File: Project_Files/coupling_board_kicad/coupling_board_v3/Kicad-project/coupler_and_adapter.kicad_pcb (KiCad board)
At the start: 2 copper layers, 98.8 x 70 mm, 95 parts, among them IC1 ISO6741DWR, IC2 ISO6740FDWR, IC3 ISO6740FDWR, J1 Conn_02x04_Odd_Even, J1 Molex Microfit, J10 Conn_02x12_Odd_Even, J2 Conn_02x04_Odd_Even, J2 Conn_02x12_Odd_Even, J3 Conn_02x04_Odd_Even, J3 Molex6, J4 Conn_02x12_Odd_Even, J5 DB25_Socket, J6 DB25_Socket, J7 Molex Microfit, J8 Molex Microfit, J9 Molex Microfit

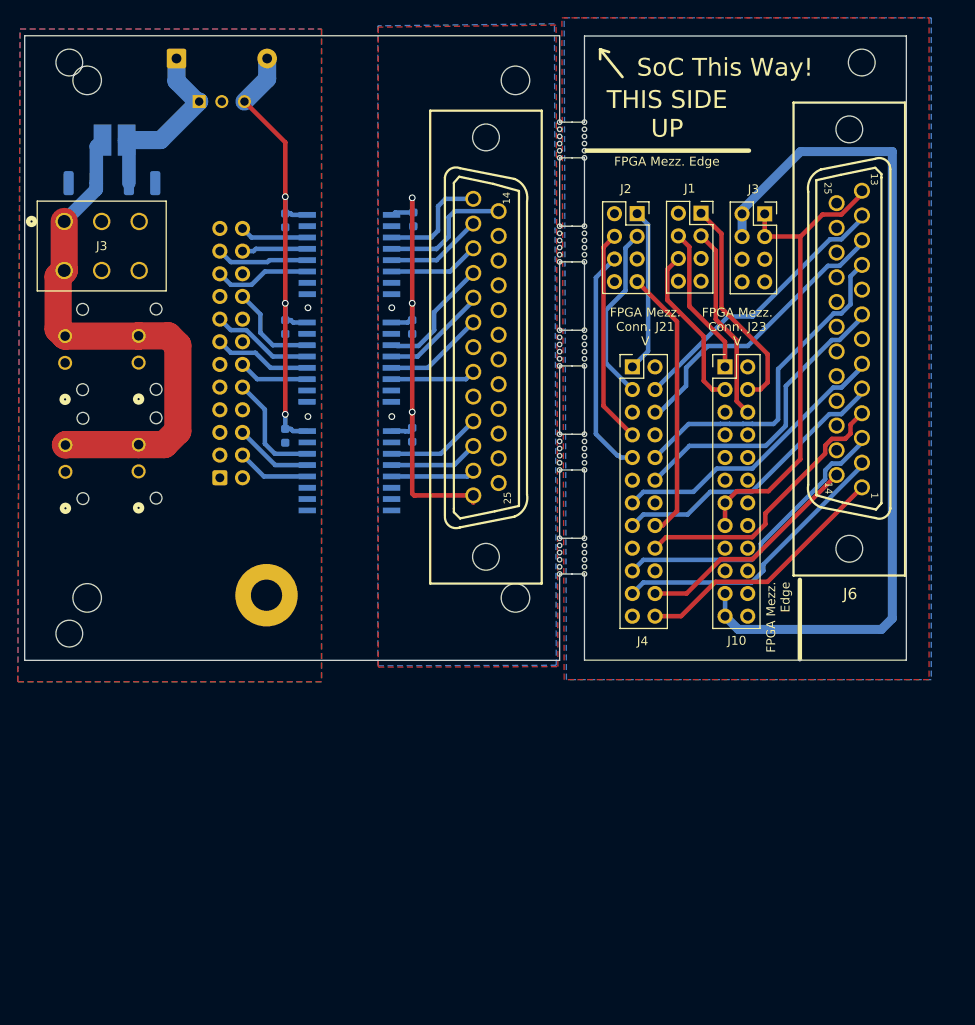
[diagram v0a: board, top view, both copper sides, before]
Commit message: Updated design files
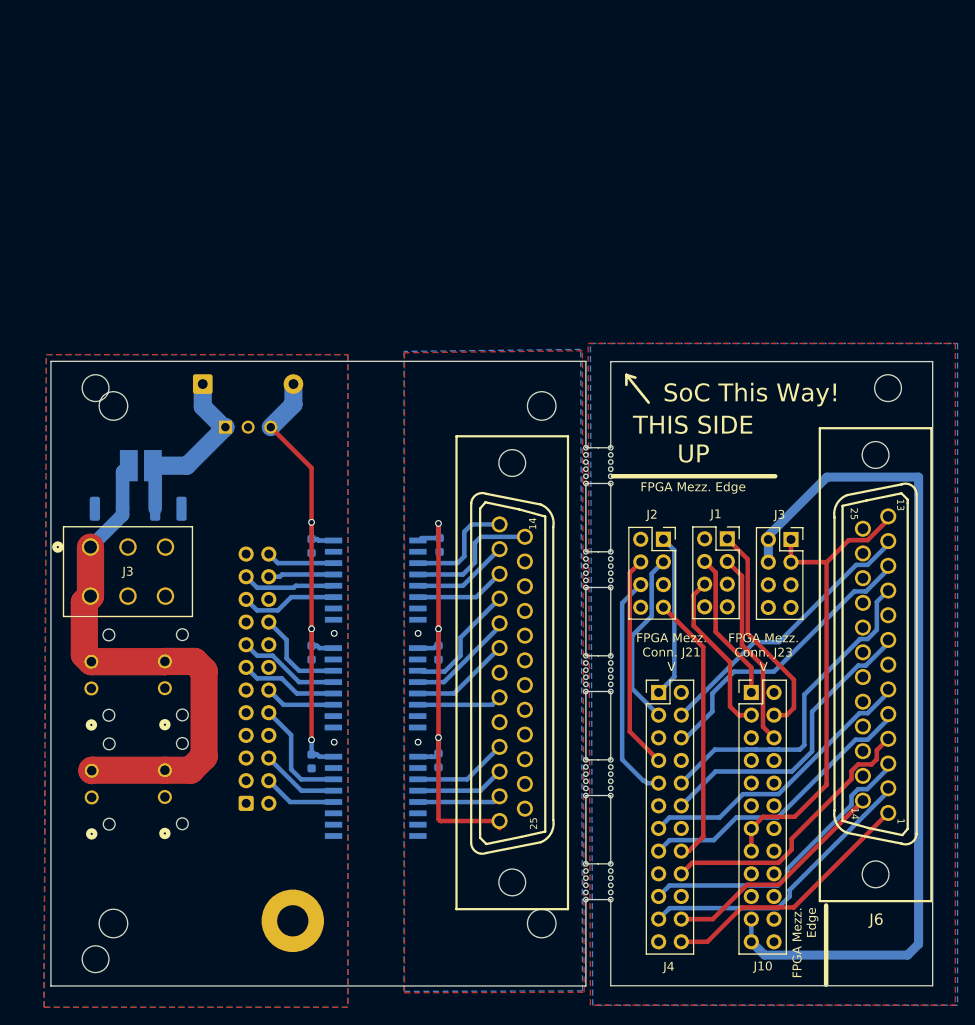
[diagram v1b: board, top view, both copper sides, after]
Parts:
- moved C7 36.6 mm to (108.4, 73.0)
- moved C9 36.6 mm to (115.2, 73.0)
- moved J3 36.6 mm to (106.5, 77.3)
- moved J5 36.6 mm to (153.7, 91.4)
- moved J7 36.6 mm to (114.5, 91.6)
- moved KiKit_MB_1_2 36.6 mm to (164.8, 69.4)
- moved KiKit_MB_2_2 36.6 mm to (164.8, 81.0)
- moved KiKit_MB_2_3 36.6 mm to (164.8, 80.2)
- moved KiKit_MB_3_3 36.6 mm to (164.8, 91.9)
- moved KiKit_MB_6_5 36.6 mm to (162.0, 69.4)
- moved KiKit_MB_7_4 36.6 mm to (162.0, 80.2)
- moved KiKit_MB_7_5 36.6 mm to (162.0, 81.0)
- moved KiKit_MB_8_4 36.6 mm to (162.0, 91.9)
- moved C1 36.6 mm to (145.5, 101.2)
- moved C3 36.6 mm to (145.6, 77.1)
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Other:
- outline, holes or cut-outs redrawn
